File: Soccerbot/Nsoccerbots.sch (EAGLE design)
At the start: 59 parts, among them X1 NXT-SOCKET, X2 NXT-SOCKET, X3 NXT-SOCKET, X4 NXT-SOCKET

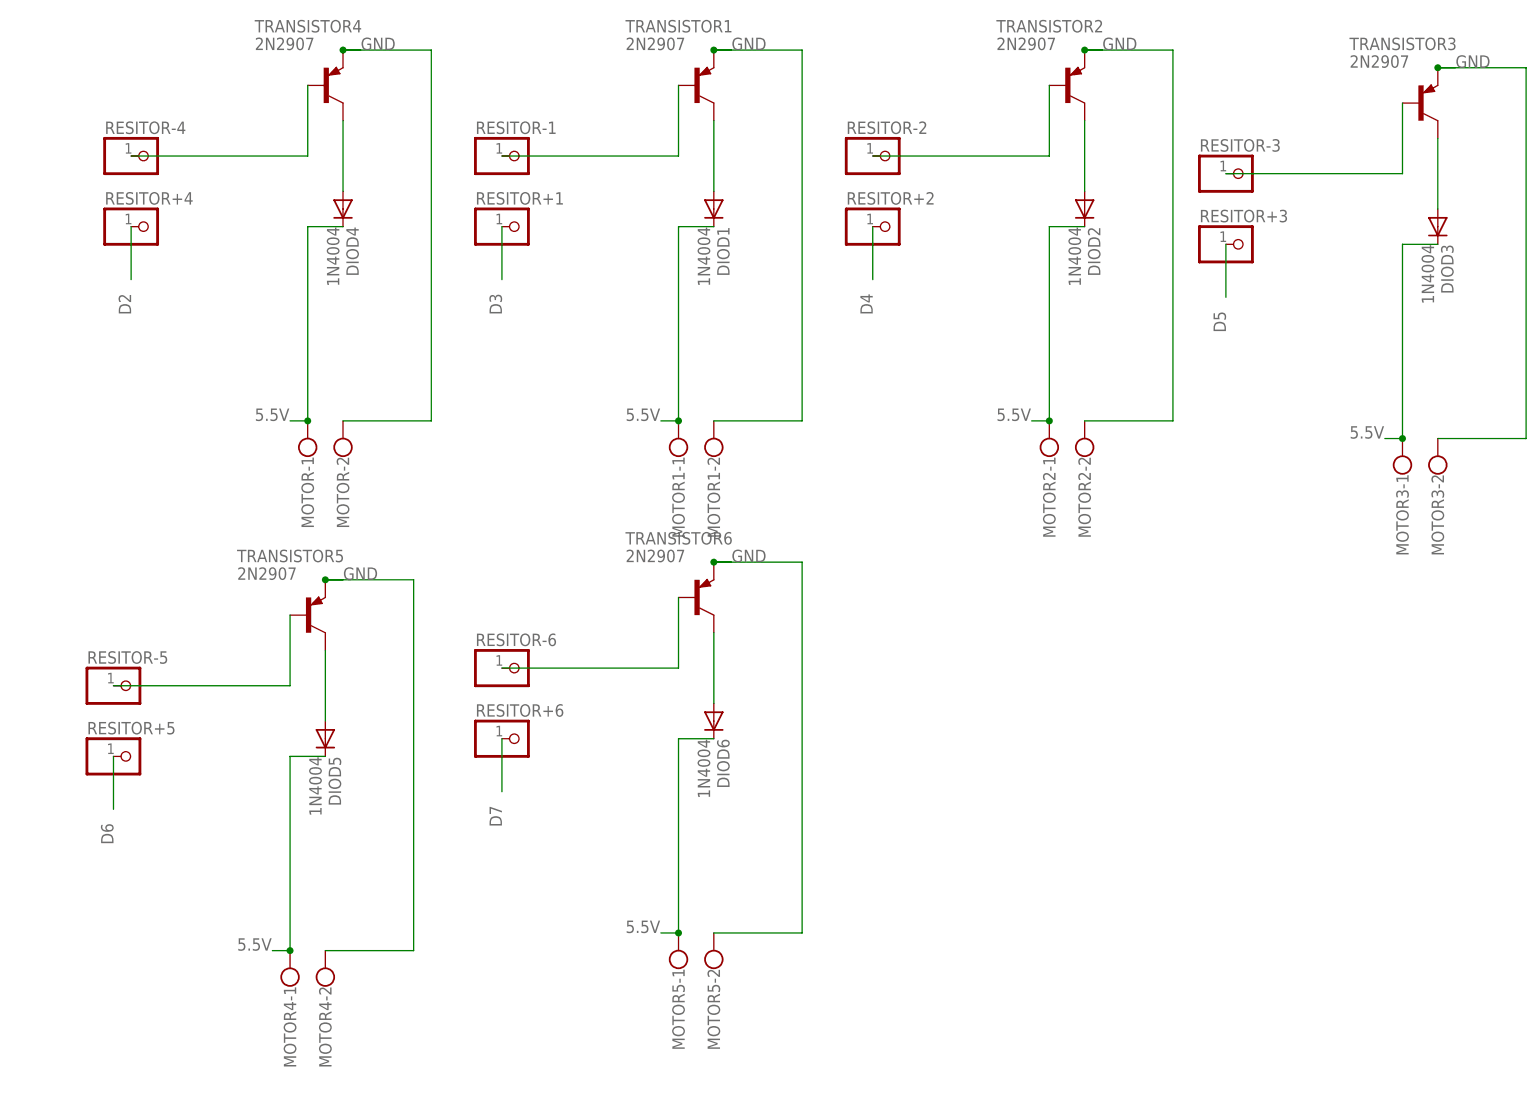
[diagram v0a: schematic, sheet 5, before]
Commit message: Z
z
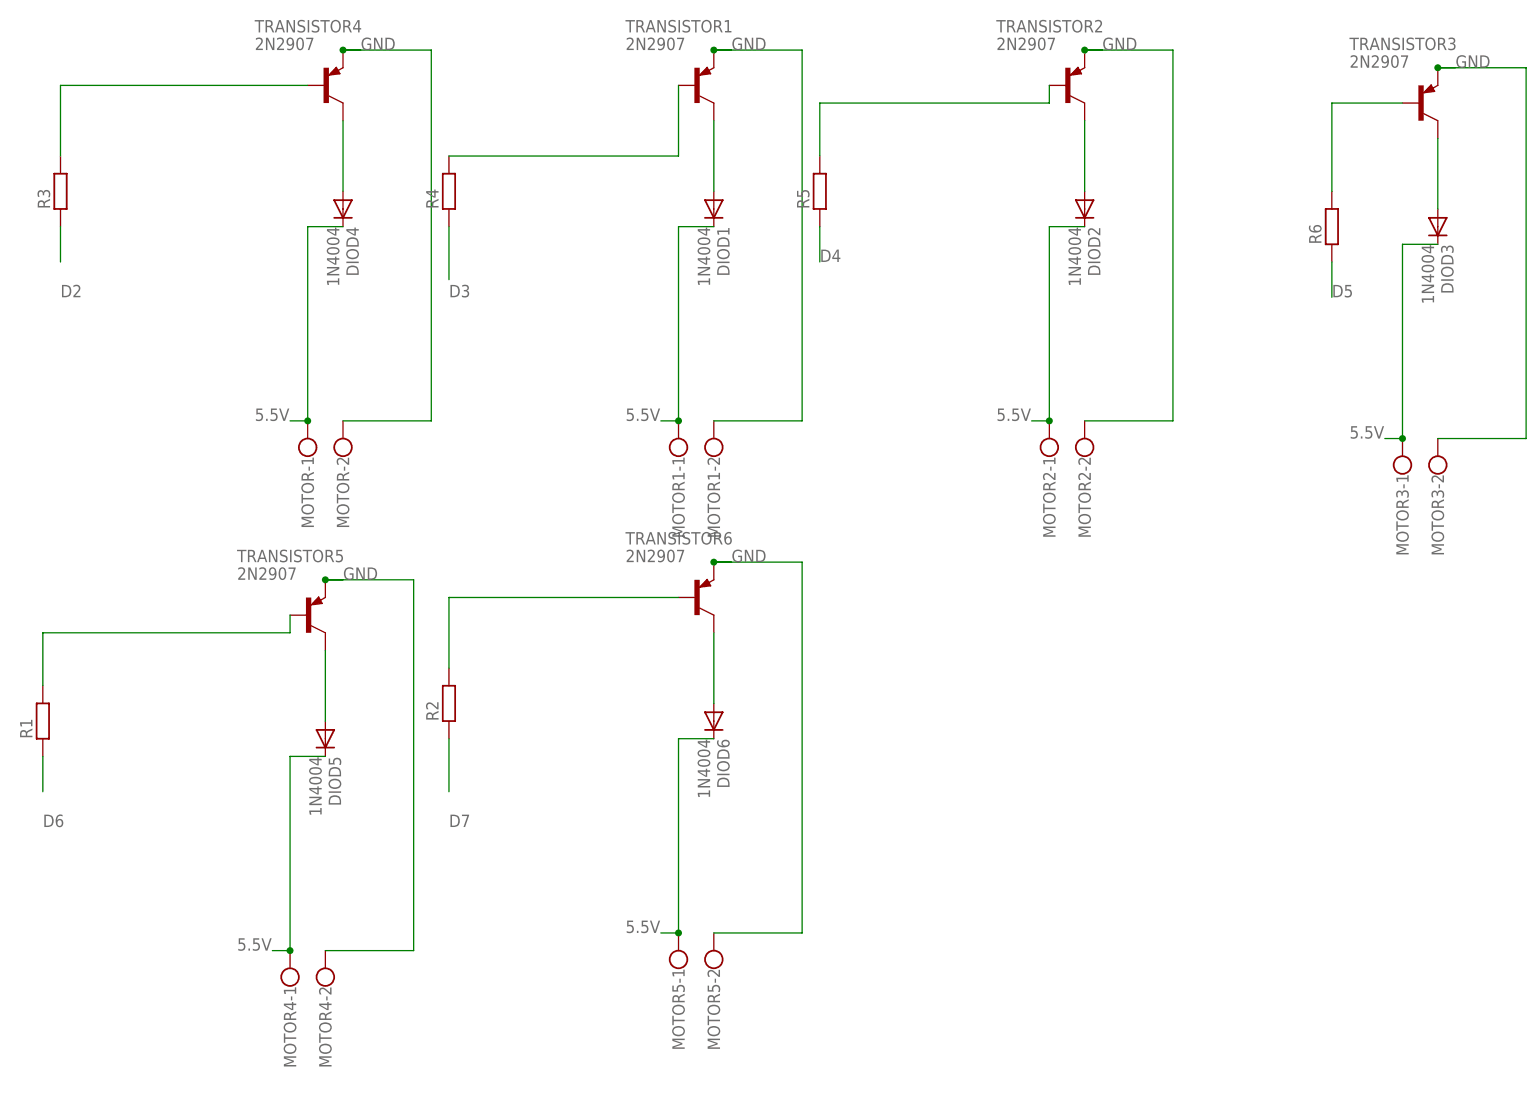
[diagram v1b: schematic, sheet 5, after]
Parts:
- removed RESITOR+1, RESITOR+2, RESITOR+3, RESITOR+4, RESITOR+5, RESITOR+6, RESITOR-1, RESITOR-2, RESITOR-3, RESITOR-4, RESITOR-5, RESITOR-6: (no value), adafruit:PINHD-1X1
- added R1, R2, R3, R4, R5, R6: (no value), BaseApp:RESISTOR
- B1: MPN (none) -> A000067; OC_NEWARK unknown -> 45W6205
- BATERY, ESC1P, ESC2P, ESC3P, ESC4P, ESC5P, ESC6P, MOTOR, MOTOR1, MOTOR2, MOTOR3, MOTOR4, MOTOR5: MPN (none) -> MA522-500M02; OC_NEWARK (none) -> 04R6830
- DIOD1, DIOD2, DIOD3, DIOD4, DIOD5, DIOD6: MPN (none) -> 1N4004-T; OC_NEWARK (none) -> 12T2303
- IMU2, IR1, IR2, IR3, IR4, IR5, IR6, JP1, JP2: OC_NEWARK (none) -> unknown
- TRANSISTOR1, TRANSISTOR2, TRANSISTOR3, TRANSISTOR4, TRANSISTOR5, TRANSISTOR6: MPN (none) -> PN2222ATF; OC_NEWARK (none) -> 29X6831
- X1, X2, X3, X4: MPN (none) -> RJE01-660-01; OC_NEWARK (none) -> 01M6133
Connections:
- net D2: now also R3.1; no longer RESITOR+4.1
- net D3: now also R4.1; no longer RESITOR+1.1
- net D4: now also R5.1; no longer RESITOR+2.1
- net D5: now also R6.1; no longer RESITOR+3.1
- net D6: now also R1.1; no longer RESITOR+5.1
- net D7: now also R2.1; no longer RESITOR+6.1
- net N$1: now also R4.2; no longer RESITOR-1.1
- net N$12: now also R2.2; no longer RESITOR-6.1
- net N$3: now also R3.2; no longer RESITOR-4.1
- net N$5: now also R5.2; no longer RESITOR-2.1
- net N$7: now also R6.2; no longer RESITOR-3.1
- net N$9: now also R1.2; no longer RESITOR-5.1
